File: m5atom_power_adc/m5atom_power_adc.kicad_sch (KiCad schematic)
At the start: 66 parts, among them J1 USB_C_Receptacle_USB2.0_14P, J2 GROVE-CONNECTOR, J3 Conn_01x04_Pin, J4 Conn_01x02, J5 Conn_01x02, J6 Conn_01x02, J7 Conn_01x02, Q1 AO3401A, Q2 MMBT2222A, Q3 MMBT2222A, SW1 Boot, SW2 Reset, U1 LM2596S-5, U2 ESP32-S3-MINI-1, U3 AMS1117-3.3, U4 ADS1115IDGS, U5 AMS1117-3.3

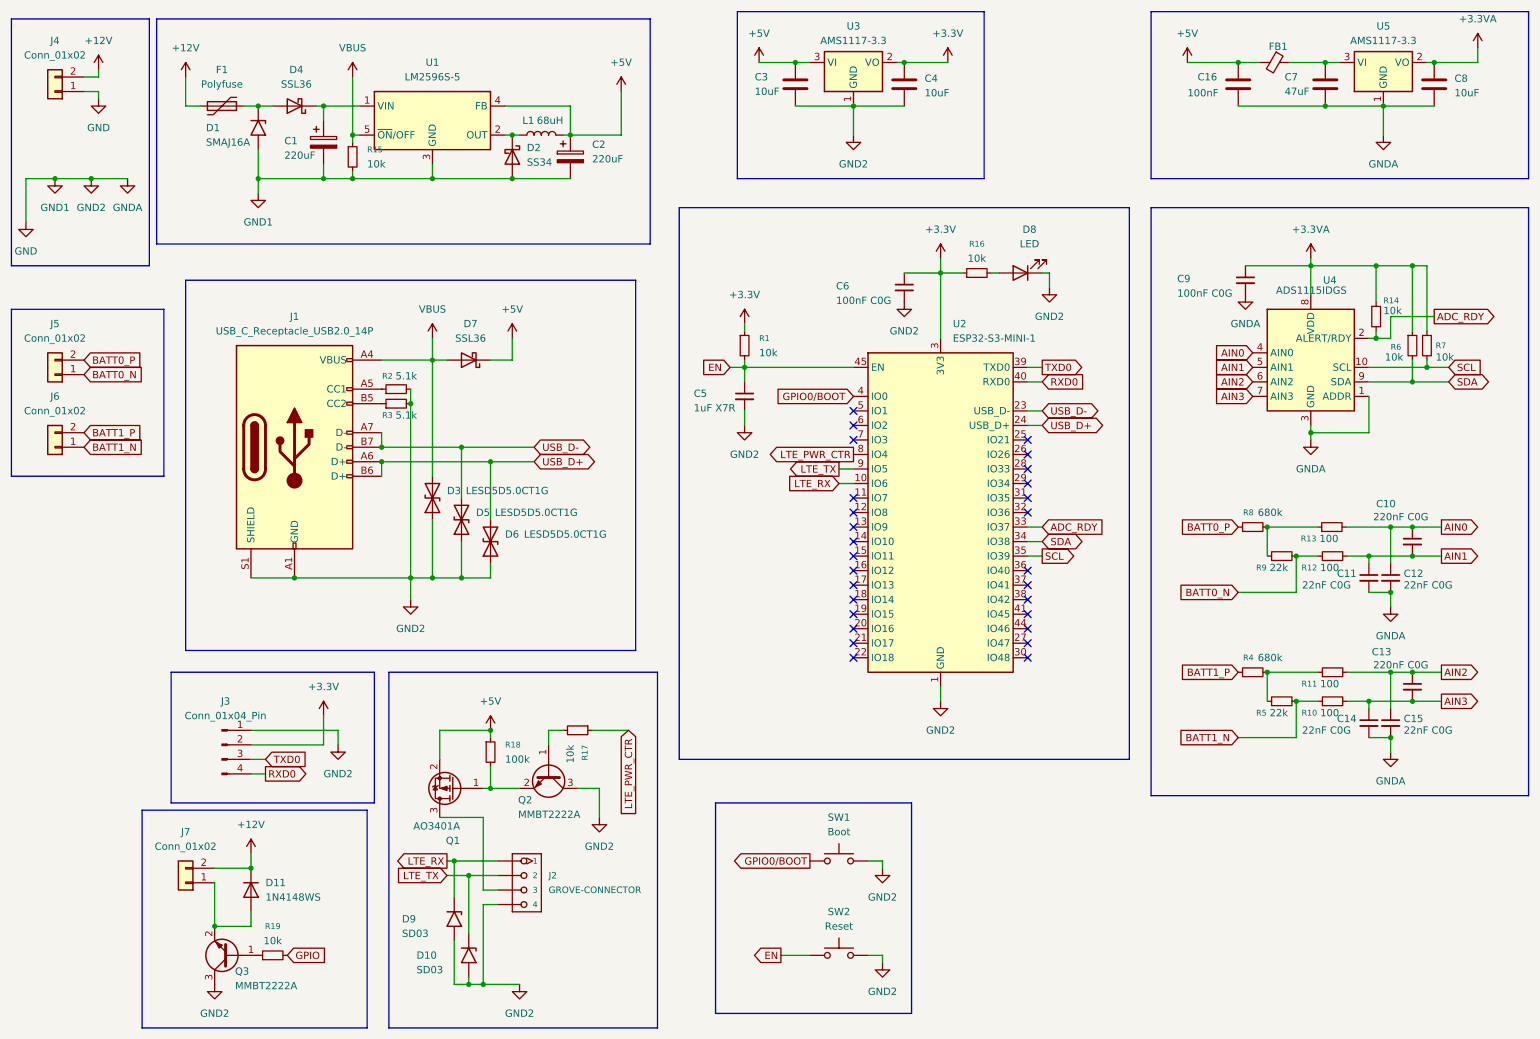
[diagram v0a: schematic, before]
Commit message: fix: いろいろ更新
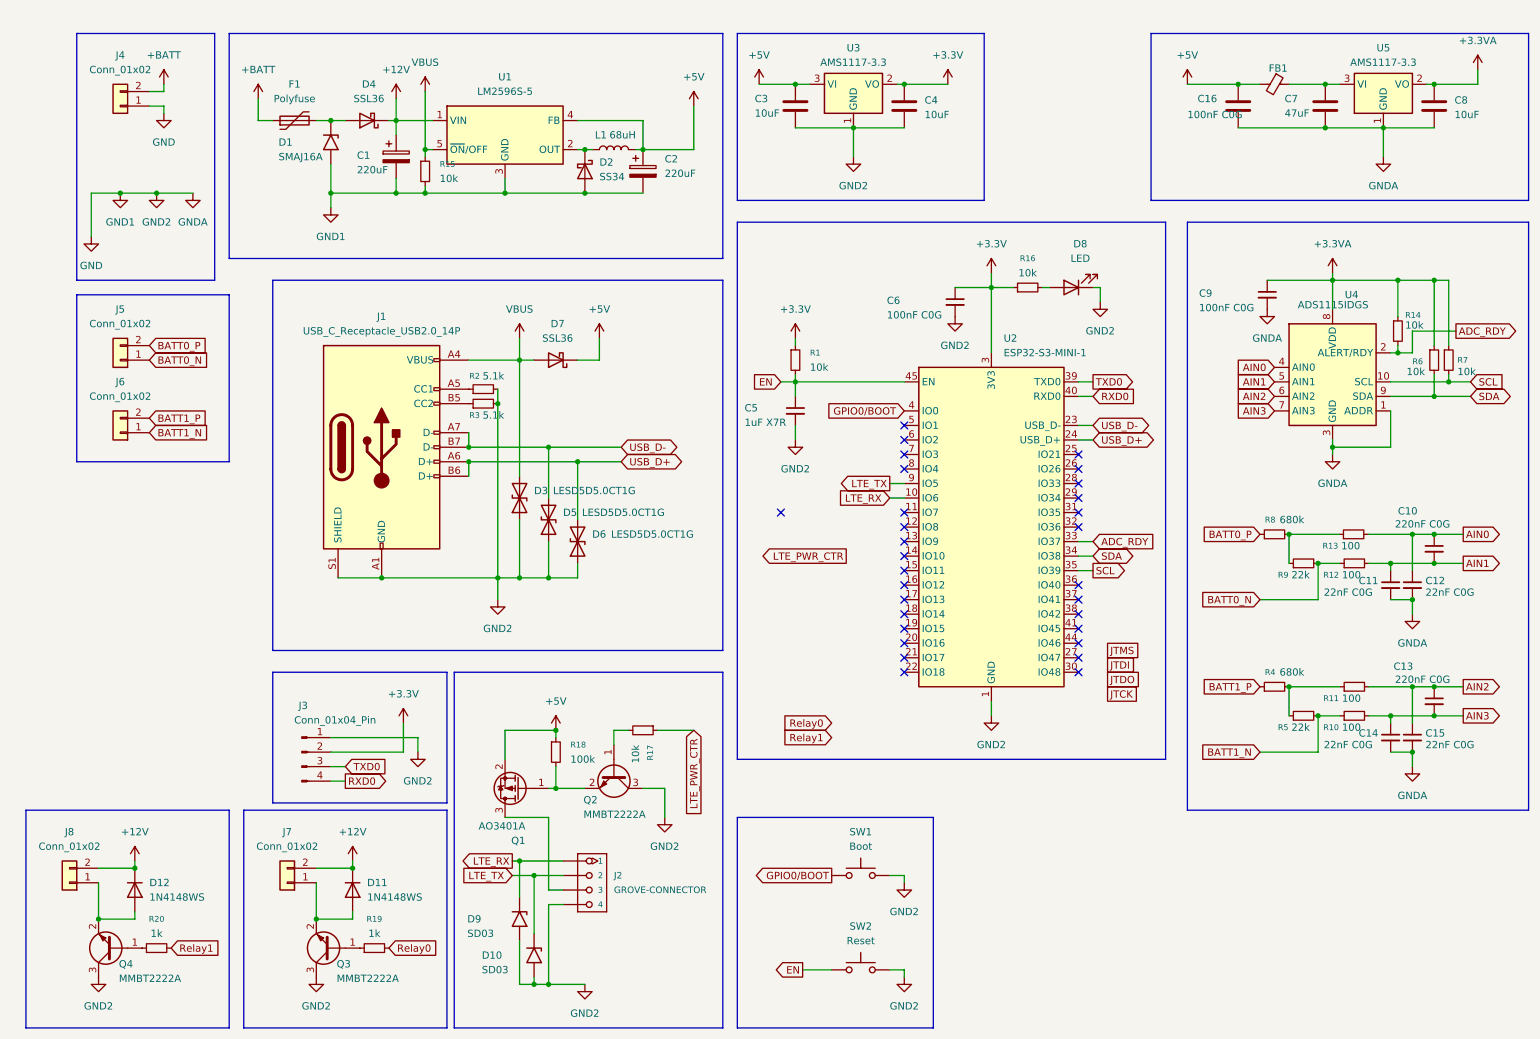
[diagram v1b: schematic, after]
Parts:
- added D12: 1N4148WS, Diode_SMD:D_SOD-323, symbol Diode:1N4148WS
- added J8: Conn_01x02, symbol Connector_Generic:Conn_01x02
- added Q4: MMBT2222A, Package_TO_SOT_SMD:SOT-23, symbol Transistor_BJT:MMBT2222A
- added R20: 1k, symbol Device:R_Small
- C1: footprint (none) -> Capacitor_SMD:CP_Elec_10x10; JLC (none) -> C125976; JLC_Num (none) -> C125976
- C16: value 100nF -> 100nF C0G; footprint (none) -> Capacitor_SMD:C_1206_3216Metric; JLC_Num (none) -> C2168319
- C2: footprint (none) -> Capacitor_SMD:CP_Elec_10x10; JLC_Num (none) -> C125976
- C6, C9: footprint (none) -> Capacitor_SMD:C_1206_3216Metric; JLC_Num (none) -> C2168319
- D1: footprint Diode_SMD:D_SMA -> Diode_SMD:D_SMB; JLC_Num (none) -> C19077571
- D10, D9: footprint Diode_SMD:D_SMA -> Diode_SMD:D_SOD-323; JLC_Num (none) -> C502526
- D11: JLC_Num (none) -> C2128
- D2: JLC_Num (none) -> C8678
- D4, D7: footprint (none) -> Diode_SMD:D_SMA; JLC_Num (none) -> C28646286
- R19: value 10k -> 1k
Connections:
- net +12V: now also C1.1, D4.1 (K), U1.1 (VIN), D12.1 (K), J8.2 (Pin_2); no longer F1.1, J4.2 (Pin_2)
- net GND: now also Q4.3 (C)
- net LTE_PWR_CTR: no longer U2.8 (IO4)
- net GPIO renamed Relay0
- new net: Q4.1 (B), R20.1
- new net: D12.2 (A), J8.1 (Pin_1), Q4.2 (E)
- new net +BATT: F1.1, J4.2 (Pin_2)
- new net Relay1: R20.2
- no-connect marks 28 -> 30
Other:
- moved on the sheet: C1, C10, C11, C12, C13, C14, C15, C16, C2, C3, C4, C5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
